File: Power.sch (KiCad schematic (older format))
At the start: 10 parts, among them U7 KF50BD-TR, U8 LM3940IMP-3.3

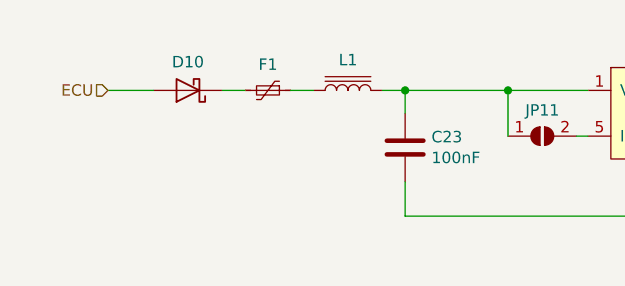
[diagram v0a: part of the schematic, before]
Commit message: Start routing
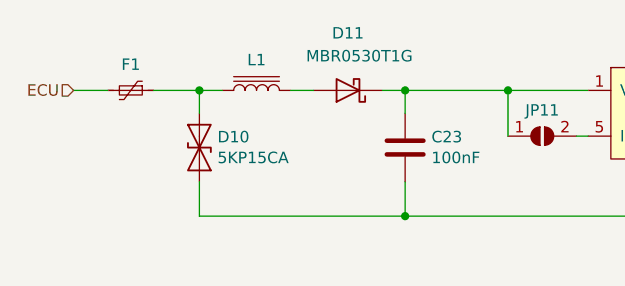
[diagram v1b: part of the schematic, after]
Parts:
- added D10: 5KP15CA, Diode_THT:D_5KP_P10.16mm_Horizontal, symbol Device:D_TVS
- L1: footprint (none) -> Inductor_SMD:L_1206_3216Metric
- renumbered D10 to D11
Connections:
- net ECU: now also F1.2; no longer D11.2 (A)
- net GND: now also D10.2 (A2)
- net at C23.1, JP11.1 (A), U7.1 (Vo): now also D11.1 (K); no longer L1.2
- net at F1.1, L1.1: now also D10.1 (A1)
- new net: D11.2 (A), L1.2
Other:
- moved on the sheet: D11, F1, L1
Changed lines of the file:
@@
 Comment4 ""
 $EndDescr
-Text HLabel 1800 2700 0    50   Input ~ 0
+Text HLabel 1650 2700 0    50   Input ~ 0
 ECU
 $Comp
@@
 L Device:L_Core_Iron L1
 U 1 1 600A9E46
-P 2850 2700
-F 0 "L1" V 2983 2700 50  0000 C CNN
-F 1 "L_Core_Iron" V 2984 2700 50  0001 C CNN
-F 2 "" H 2850 2700 50  0001 C CNN
-F 3 "~" H 2850 2700 50  0001 C CNN
-F 4 "MOUNT" H 2850 2700 50  0001 C CNN "Mount"
-F 5 "SMD" H 2850 2700 50  0001 C CNN "MountType"
-F 6 "-" H 2850 2700 50  0001 C CNN "Manufacturer"
-	1    2850 2700
+P 2450 2700
+F 0 "L1" V 2583 2700 50  0000 C CNN
+F 1 "L_Core_Iron" V 2584 2700 50  0001 C CNN
+F 2 "Inductor_SMD:L_1206_3216Metric" H 2450 2700 50  0001 C CNN
+F 3 "~" H 2450 2700 50  0001 C CNN
+F 4 "MOUNT" H 2450 2700 50  0001 C CNN "Mount"
+F 5 "SMD" H 2450 2700 50  0001 C CNN "MountType"
+F 6 "-" H 2450 2700 50  0001 C CNN "Manufacturer"
+	1    2450 2700
 	0    -1   -1   0
 $EndComp
@@
 	3100 2700 3100 2800
 Connection ~ 3100 2700
-Wire Wire Line
-	1800 2700 2000 2700
 Wire Wire Line
 	4800 2700 5000 2700
@@
 	7200 2700 7300 2700
 $Comp
-L Device:D_Schottky D10
+L Device:D_Schottky D11
 U 1 1 600DD919
-P 2150 2700
-F 0 "D10" H 2150 2576 50  0000 C CNN
-F 1 "MBR0530T1G" H 2150 2575 50  0001 C CNN
-F 2 "Diode_SMD:D_SOD-123" H 2150 2700 50  0001 C CNN
-F 3 "https://datasheet.lcsc.com/szlcsc/ON-Semicon-ON-MBR0530T1G_C82046.pdf" H 2150 2700 50  0001 C CNN
-F 4 "30V 500mA 430mV @ 500mA SOD-123 Schottky Barrier Diodes" H 2150 2700 50  0001 C CNN "Description"
-F 5 "ON Semiconductor" H 2150 2700 50  0001 C CNN "Manufacturer"
-F 6 "MOUNT" H 2150 2700 50  0001 C CNN "Mount"
-F 7 "SMD" H 2150 2700 50  0001 C CNN "MountType"
-F 8 "MBR0530T1G" H 2150 2700 50  0001 C CNN "PartNumber"
-	1    2150 2700
+P 2850 2700
+F 0 "D11" H 2850 2450 50  0000 C CNN
+F 1 "MBR0530T1G" H 2800 2550 50  0000 C CNN
+F 2 "Diode_SMD:D_SOD-123" H 2850 2700 50  0001 C CNN
+F 3 "https://datasheet.lcsc.com/szlcsc/ON-Semicon-ON-MBR0530T1G_C82046.pdf" H 2850 2700 50  0001 C CNN
+F 4 "30V 500mA 430mV @ 500mA SOD-123 Schottky Barrier Diodes" H 2850 2700 50  0001 C CNN "Description"
+F 5 "ON Semiconductor" H 2850 2700 50  0001 C CNN "Manufacturer"
+F 6 "MOUNT" H 2850 2700 50  0001 C CNN "Mount"
+F 7 "SMD" H 2850 2700 50  0001 C CNN "MountType"
+F 8 "MBR0530T1G" H 2850 2700 50  0001 C CNN "PartNumber"
+	1    2850 2700
 	-1   0    0    1
 $EndComp
@@
 L Device:Polyfuse_Small F1
 U 1 1 600DEBDF
-P 2500 2700
-F 0 "F1" V 2387 2700 50  0000 C CNN
-F 1 "1206L025YR" V 2386 2700 50  0001 C CNN
-F 2 "Fuse:Fuse_1206_3216Metric" H 2550 2500 50  0001 L CNN
-F 3 "https://datasheet.lcsc.com/szlcsc/Littelfuse-1206L025YR_C99561.pdf" H 2500 2700 50  0001 C CNN
-F 4 "Polymeric 16V 500mA 100ms 750mΩ 1206 PTC Resettable Fuses RoHS" H 2500 2700 50  0001 C CNN "Description"
-F 5 "Littelfuse" H 2500 2700 50  0001 C CNN "Manufacturer"
-F 6 "MOUNT" H 2500 2700 50  0001 C CNN "Mount"
-F 7 "SMD" H 2500 2700 50  0001 C CNN "MountType"
-F 8 "1206L025YR" H 2500 2700 50  0001 C CNN "PartNumber"
-	1    2500 2700
+P 1900 2700
+F 0 "F1" V 1787 2700 50  0000 C CNN
+F 1 "1206L025YR" V 1786 2700 50  0001 C CNN
+F 2 "Fuse:Fuse_1206_3216Metric" H 1950 2500 50  0001 L CNN
+F 3 "https://datasheet.lcsc.com/szlcsc/Littelfuse-1206L025YR_C99561.pdf" H 1900 2700 50  0001 C CNN
+F 4 "Polymeric 16V 500mA 100ms 750mΩ 1206 PTC Resettable Fuses RoHS" H 1900 2700 50  0001 C CNN "Description"
+F 5 "Littelfuse" H 1900 2700 50  0001 C CNN "Manufacturer"
+F 6 "MOUNT" H 1900 2700 50  0001 C CNN "Mount"
+F 7 "SMD" H 1900 2700 50  0001 C CNN "MountType"
+F 8 "1206L025YR" H 1900 2700 50  0001 C CNN "PartNumber"
+	1    1900 2700
 	0    1    1    0
 $EndComp
 Wire Wire Line
-	2300 2700 2400 2700
-Wire Wire Line
-	2600 2700 2700 2700
+	2000 2700 2200 2700
+$Comp
+L Device:D_TVS D10
+U 1 1 600F6140
+P 2200 2950
+F 0 "D10" V 2154 3029 50  0000 L CNN
+F 1 "5KP15CA" V 2245 3029 50  0000 L CNN
+F 2 "Diode_THT:D_5KP_P10.16mm_Horizontal" H 2200 2950 50  0001 C CNN
+F 3 "https://m.littelfuse.com/~/media/electronics/datasheets/tvs_diodes/littelfuse_tvs_diode_5kp_datasheet.pdf.pdf" H 2200 2950 50  0001 C CNN
+	1    2200 2950
+	0    1    1    0
+$EndComp
+Wire Wire Line
+	2700 2700 2600 2700
+Wire Wire Line
+	2200 2700 2200 2800
+Wire Wire Line
+	2200 3100 2200 3250
+Connection ~ 3100 3250
+Connection ~ 2200 2700
+Wire Wire Line
+	2200 2700 2300 2700
+Wire Wire Line
+	1650 2700 1800 2700
+Wire Wire Line
+	2200 3250 3100 3250
 $EndSCHEMATC
